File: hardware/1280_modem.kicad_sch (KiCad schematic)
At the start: 84 parts, among them IC1 SX1281IMLTRT, IC2 SKY65383-11, IC3 TJA1462AT_0Z, J2 Conn_Coaxial, J2 jst gh 4, J5 jst gh 6, J8 USB_C_Receptacle_USB2.0, J9 jst_sh 6, U13 STM32U575CGTx, U2 TPS7A20285PDBVR, U2 USBLC6-2SC6, U4 TPS7A2450DBVR, Y1 48MHz, Y1 52MHz

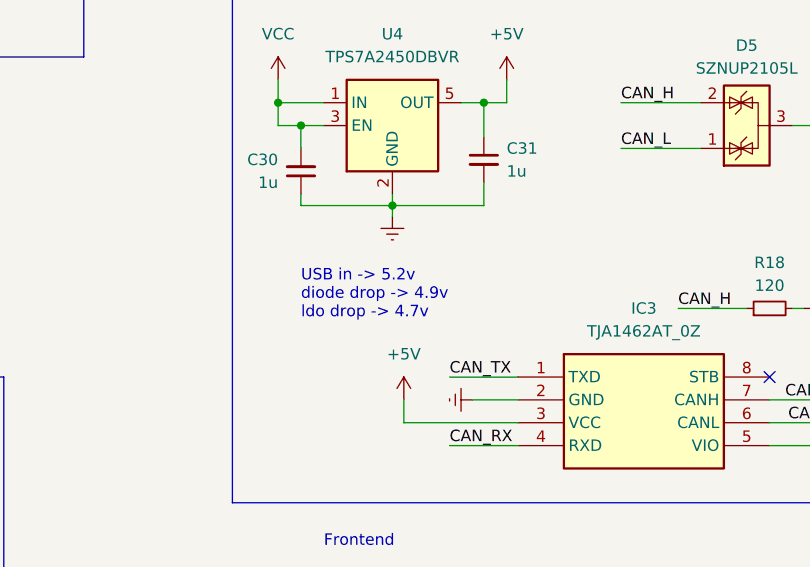
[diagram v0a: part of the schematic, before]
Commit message: add pdf
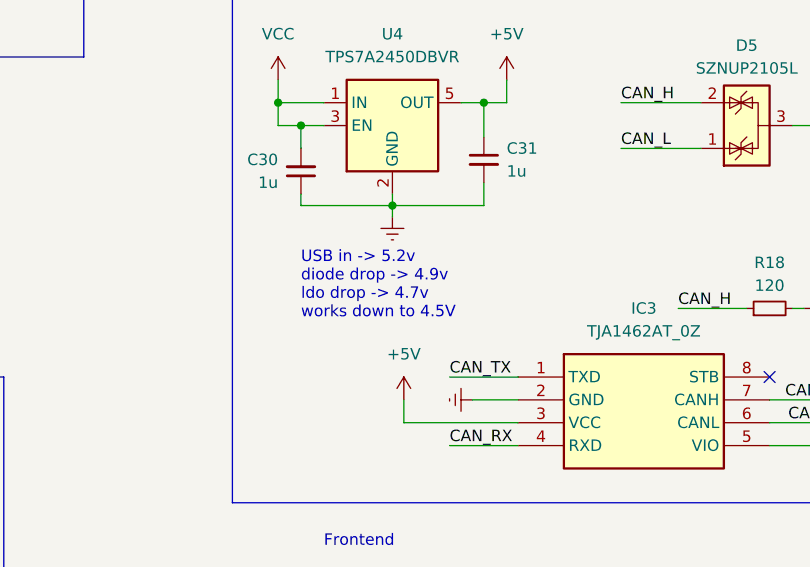
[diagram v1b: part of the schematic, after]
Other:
- note added: "USB in -> 5.2v diode drop -> 4.9v ldo drop -> 4.7v works down to 4.5V"
- note removed: "USB in -> 5.2v diode drop -> 4.9v ldo drop -> 4.7v"
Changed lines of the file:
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@@
     (effects (font (size 1.27 1.27)) (justify left bottom))
   )
-  (text "USB in -> 5.2v\ndiode drop -> 4.9v\nldo drop -> 4.7v\n"
+  (text "USB in -> 5.2v\ndiode drop -> 4.9v\nldo drop -> 4.7v\nworks down to 4.5V"
     (at 180.34 173.99 0)
     (effects (font (size 1.27 1.27)) (justify left bottom))
